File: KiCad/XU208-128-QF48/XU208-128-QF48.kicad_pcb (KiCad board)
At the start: 2 copper layers, 1 part, among them U1 XU208-128-QF48-I10

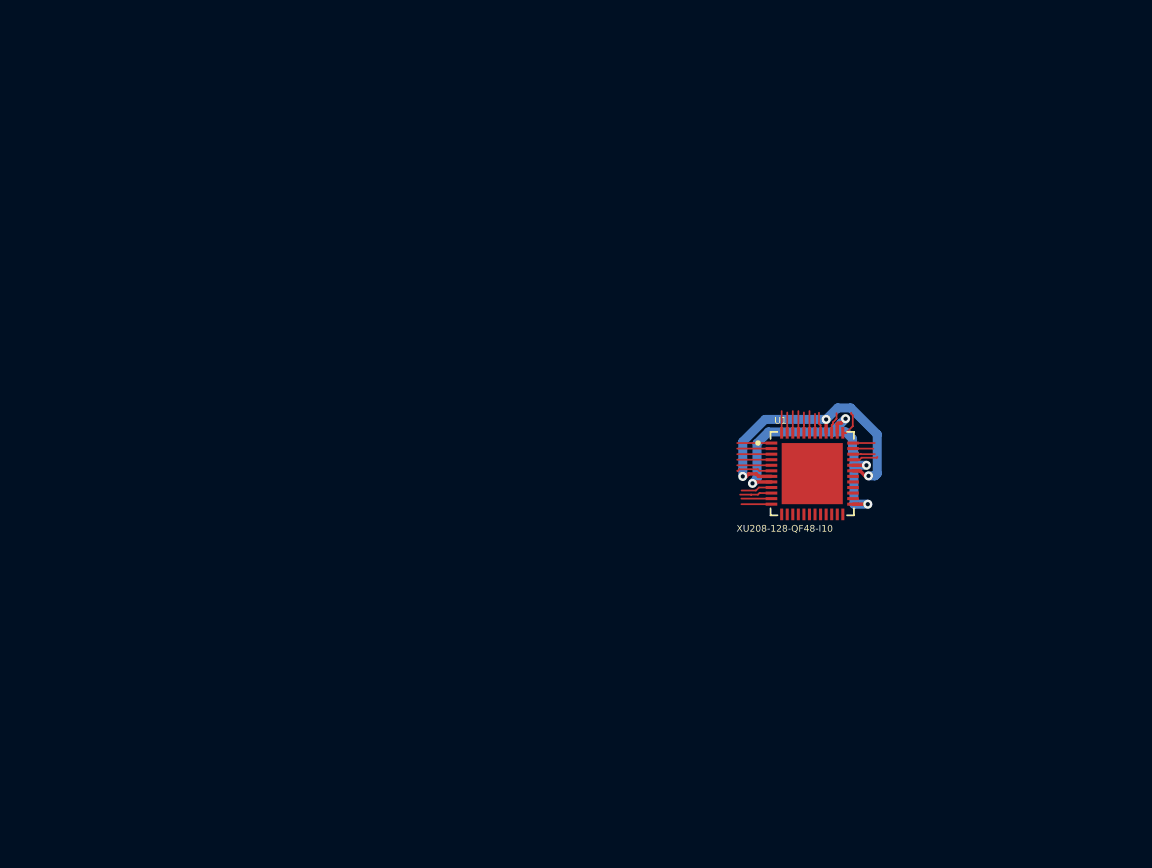
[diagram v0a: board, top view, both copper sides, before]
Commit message: Schematic and board
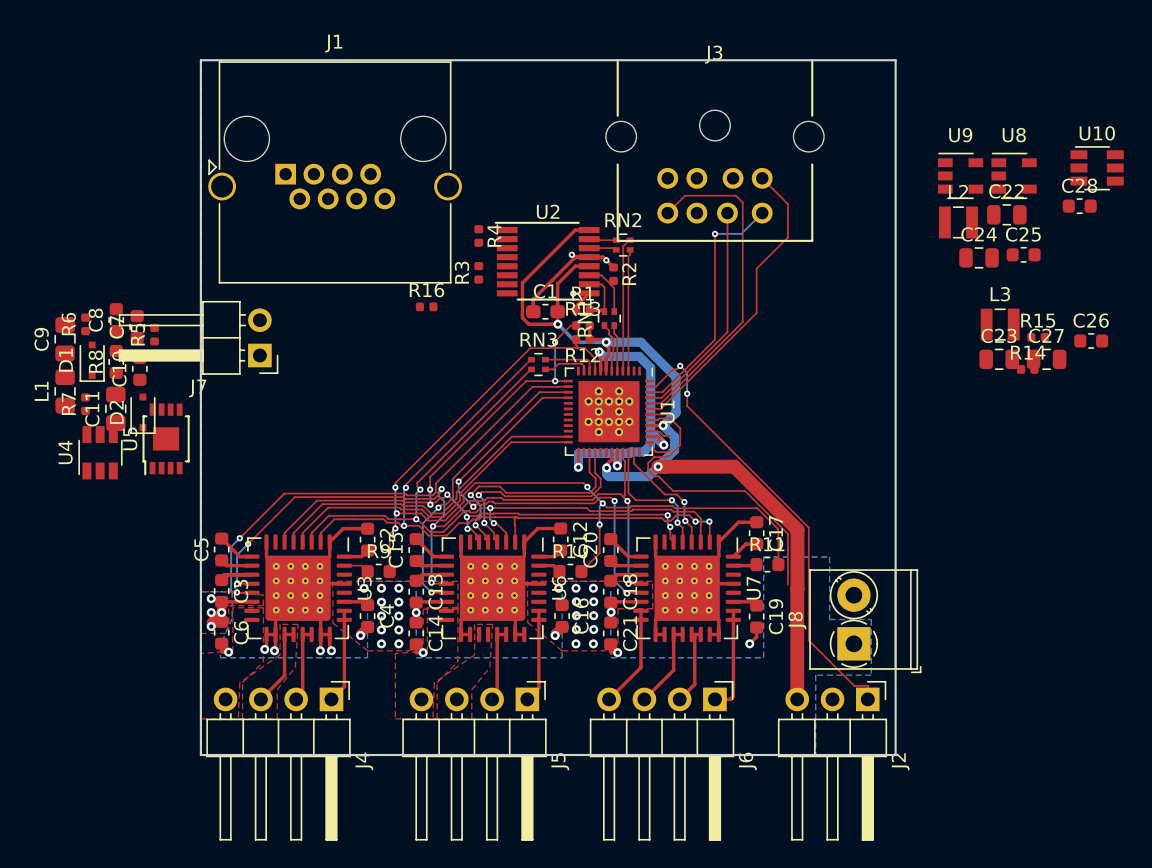
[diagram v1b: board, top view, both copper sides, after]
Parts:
- added C1: 100nF, Capacitor_SMD:C_0603_1608Metric_Pad1.05x0.95mm_HandSolder, F.Cu at (104.8, 78.1)
- added C10: 1uF, Capacitor_SMD:C_0603_1608Metric, F.Cu at (75.6, 82.2)
- added C11: 4u7, Capacitor_SMD:C_0805_2012Metric_Pad1.15x1.40mm_HandSolder, F.Cu at (73.9, 85.1)
- added C12: 100nF, Capacitor_SMD:C_0603_1608Metric, F.Cu at (105.9, 94.5)
- added C13: 220nF, Capacitor_SMD:C_0603_1608Metric, F.Cu at (95.5, 98.2)
- added C14: 100nF, Capacitor_SMD:C_0603_1608Metric, F.Cu at (95.5, 101.2)
- added C15: 100nF, Capacitor_SMD:C_0603_1608Metric, F.Cu at (95.5, 95.2)
- added C16: 100nF, Capacitor_SMD:C_0603_1608Metric, F.Cu at (106.0, 100.0)
- added C17: 100nF, Capacitor_SMD:C_0603_1608Metric, F.Cu at (120.0, 94.0)
- added C18: 220nF, Capacitor_SMD:C_0603_1608Metric, F.Cu at (109.5, 98.2)
- added C19: 100nF, Capacitor_SMD:C_0603_1608Metric, F.Cu at (120.0, 100.0)
- added C2: 100nF, Capacitor_SMD:C_0603_1608Metric, F.Cu at (92.0, 94.5)
- added C20: 100nF, Capacitor_SMD:C_0603_1608Metric, F.Cu at (109.5, 95.2)
- added C21: 100nF, Capacitor_SMD:C_0603_1608Metric, F.Cu at (109.5, 101.2)
- added C22: 22uF, Capacitor_SMD:C_0805_2012Metric, F.Cu at (138.0, 71.1)
- added C23: 2u2F, Capacitor_SMD:C_0805_2012Metric, F.Cu at (137.5, 81.5)
- added C24: 2u2F, Capacitor_SMD:C_0805_2012Metric, F.Cu at (136.0, 74.2)
- added C25: 100n, Capacitor_SMD:C_0603_1608Metric, F.Cu at (139.2, 74.0)
- added C26: 100n, Capacitor_SMD:C_0603_1608Metric, F.Cu at (144.1, 80.2)
- added C27: 22uF, Capacitor_SMD:C_0805_2012Metric, F.Cu at (140.9, 81.5)
- added C28: 470p, Capacitor_SMD:C_0603_1608Metric, F.Cu at (143.2, 70.5)
- added C3: 220nF, Capacitor_SMD:C_0603_1608Metric, F.Cu at (81.5, 98.2)
- added C4: 100nF, Capacitor_SMD:C_0603_1608Metric, F.Cu at (92.0, 100.0)
- added C5: 100nF, Capacitor_SMD:C_0603_1608Metric, F.Cu at (81.5, 95.2)
- added C6: 100nF, Capacitor_SMD:C_0603_1608Metric, F.Cu at (81.5, 101.2)
- added C7: 1nF, Capacitor_SMD:C_0603_1608Metric, F.Cu at (75.4, 79.2)
- added C8: 1nF, Capacitor_SMD:C_0603_1608Metric, F.Cu at (73.9, 78.7)
- added C9: 4u7, Capacitor_SMD:C_0805_2012Metric_Pad1.15x1.40mm_HandSolder, F.Cu at (70.2, 80.1)
- added D1: SCHOTTKY_DIODE, Diode_SMD:D_SOD-323F, F.Cu at (72.2, 81.6)
- added D2: SCHOTTKY_DIODE, Diode_SMD:D_SOD-323F, F.Cu at (75.8, 85.3)
- added J1: RJ45_Shielded, Connector_RJ:RJ45_Amphenol_RJHSE5380, F.Cu at (86.1, 68.2)
- added J2: ZLIM, Connector_PinHeader_2.54mm:PinHeader_1x03_P2.54mm_Horizontal, F.Cu at (128.0, 106.0)
- added J3: Mini-DIN-8, library:MDC-278, F.Cu at (117.0, 60.0)
- added J4: Conn_01x04, Connector_PinHeader_2.54mm:PinHeader_1x04_P2.54mm_Horizontal, F.Cu at (89.4, 106.0)
- added J5: Conn_01x04, Connector_PinHeader_2.54mm:PinHeader_1x04_P2.54mm_Horizontal, F.Cu at (103.5, 106.0)
- added J6: Conn_01x04, Connector_PinHeader_2.54mm:PinHeader_1x04_P2.54mm_Horizontal, F.Cu at (117.0, 106.0)
- added J7: LED, Connector_PinHeader_2.54mm:PinHeader_1x02_P2.54mm_Horizontal, F.Cu at (84.2, 81.2)
- added J8: Screw_Terminal_01x02, TerminalBlock_Phoenix:TerminalBlock_Phoenix_PT-1,5-2-3.5-H_1x02_P3.50mm_Horizontal, F.Cu at (127.0, 102.0)
- added L1: 22uH, Capacitor_SMD:C_0805_2012Metric_Pad1.15x1.40mm_HandSolder, F.Cu at (70.2, 83.8)
- added L2: 4u7, Inductor_SMD:L_Wuerth_MAPI-2510, F.Cu at (134.5, 71.7)
- added L3: 4u7, Inductor_SMD:L_Wuerth_MAPI-2510, F.Cu at (137.5, 79.0)
- added R1: 47k, Resistor_SMD:R_0402_1005Metric, F.Cu at (107.5, 78.0)
- added R10: 33R, Resistor_SMD:R_0603_1608Metric, F.Cu at (106.6, 96.8)
- added R11: 33R, Resistor_SMD:R_0603_1608Metric, F.Cu at (120.8, 96.3)
- added R12: 3k3, Resistor_SMD:R_0402_1005Metric, F.Cu at (107.5, 80.1)
- added R13: 3k3, Resistor_SMD:R_0402_1005Metric, F.Cu at (107.5, 79.1)
- added R14: 15k, Resistor_SMD:R_0402_1005Metric, F.Cu at (139.5, 82.2)
- added R15: 10k, Resistor_SMD:R_0402_1005Metric, F.Cu at (140.3, 79.9)
- added R16: 10k, Resistor_SMD:R_0402_1005Metric, F.Cu at (96.2, 77.8)
- added R2: 47k, Resistor_SMD:R_0402_1005Metric, F.Cu at (109.7, 75.4)
- added R3: 100R, Resistor_SMD:R_0402_1005Metric, F.Cu at (100.0, 75.3)
- added R4: 100R, Resistor_SMD:R_0402_1005Metric, F.Cu at (100.0, 72.7)
- added R5: 33k, Resistor_SMD:R_0402_1005Metric, F.Cu at (76.7, 79.8)
- added R6: 33k, Resistor_SMD:R_0402_1005Metric, F.Cu at (71.7, 79.0)
- added R7: 47k, Resistor_SMD:R_0402_1005Metric, F.Cu at (71.7, 84.8)
- added R8: 1R, Resistor_SMD:R_0603_1608Metric, F.Cu at (73.9, 81.7)
- added R9: 33R, Resistor_SMD:R_0603_1608Metric, F.Cu at (92.8, 96.8)
- added RN1: 33R, Resistor_SMD:R_Array_Convex_2x0402, F.Cu at (109.4, 78.6)
- added RN2: 33R, Resistor_SMD:R_Array_Convex_2x0402, F.Cu at (110.4, 73.3)
- added RN3: 33R, Resistor_SMD:R_Array_Convex_2x0402, F.Cu at (104.3, 81.9)
- added U10: NCP308SN090T1G, Package_TO_SOT_SMD:TSOT-23-6, F.Cu at (144.5, 67.8)
- added U2: DS90LV049TMT, Package_SO:TSSOP-16_4.4x5mm_P0.65mm, F.Cu at (105.0, 74.5)
- added U3: AMIS-30543, Package_DFN_QFN:QFN-32-1EP_7x7mm_P0.65mm_EP4.7x4.7mm_ThermalVias, F.Cu at (87.0, 98.0)
- added U4: NCP308SN090T1G, Package_TO_SOT_SMD:TSOT-23-6, F.Cu at (72.8, 88.2)
- added U5: LM3407MY, Package_SO:MSOP-8-1EP_3x3mm_P0.65mm_EP1.68x1.88mm, F.Cu at (77.5, 87.2)
- added U6: AMIS-30543, Package_DFN_QFN:QFN-32-1EP_7x7mm_P0.65mm_EP4.7x4.7mm_ThermalVias, F.Cu at (101.0, 98.0)
- added U7: AMIS-30543, Package_DFN_QFN:QFN-32-1EP_7x7mm_P0.65mm_EP4.7x4.7mm_ThermalVias, F.Cu at (115.0, 98.0)
- added U8: TPS560430X3FDBVT, Package_TO_SOT_SMD:SOT-23-5, F.Cu at (138.5, 68.3)
- added U9: TPS560430XFDBVR, Package_TO_SOT_SMD:SOT-23-5, F.Cu at (134.7, 68.3)
- U1: footprint XU208-128-QF48-I10:QFN40P600X600X60-49N -> Package_DFN_QFN:QFN-48-1EP_6x6mm_P0.4mm_EP4.66x4.66mm_ThermalVias
- moved U1 15.3 mm to (109.4, 85.3), turned to 270 degrees
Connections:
- net /CLK renamed /CLK_20MHz
- net /PLL_AVDD renamed Net-(U1-Pad39)
- U1 pad 6: /L1.out0 -> /L0.out1
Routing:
- net GND: track 0.00 -> 96.8 mm, vias 0 -> 13
- net /1B: track 2.24 -> 66.2 mm, vias 0 -> 6
- net /1D: track 0.00 -> 54.6 mm, vias 0 -> 9
- net /1L: track 1.85 -> 54.1 mm, vias 0 -> 7
- net /CLK: track 0.00 -> 50.1 mm, vias 0 -> 4
- net /MOSI: track 0.00 -> 49.7 mm, vias 0 -> 4
- net +3V3: track 21.9 -> 70.4 mm, vias 3 -> 5
- net /4B1: track 0.00 -> 34.2 mm, vias 0 -> 2
- net /1N: track 1.47 -> 33.0 mm, vias 0 -> 2
- net /4B3: track 0.00 -> 31.3 mm, vias 0 -> 4
- net /4C0: track 0.00 -> 24.2 mm
- net /4C1: track 0.00 -> 23.3 mm
- net /TCK: track 1.47 -> 23.8 mm
- net /4B2: track 0.00 -> 21.5 mm, vias 0 -> 2
- net /~RST: track 1.50 -> 22.7 mm
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- added copper zone on B.Cu, net +24V
- added copper zone on F.Cu, net +24V
- added copper zone on F.Cu, net /AMIS30543A/YN
- added copper zone on F.Cu, net /AMIS30543A/YP
- added copper zone on F.Cu, net /AMIS30543B/YN
- added copper zone on F.Cu, net /AMIS30543B/YP
- added copper zone on B.Cu, net GND
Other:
- board outline added: 50 x 50 mm
- net class 24V added: clearance 0.2, trace_width 0.25, via_dia 0.65, via_drill 0.3
